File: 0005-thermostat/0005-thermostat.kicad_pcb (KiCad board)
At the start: 2 copper layers, 68.5 x 42 mm, 50 parts, among them J1 EXT_NTC, J2 OUT, J3 PWR, J4 EXT_LED, J5 EXT_P1, J6 EXT_P2, P1 22k, P2 22k, T1 BC847B, T2 BC847B, T3 BC847B

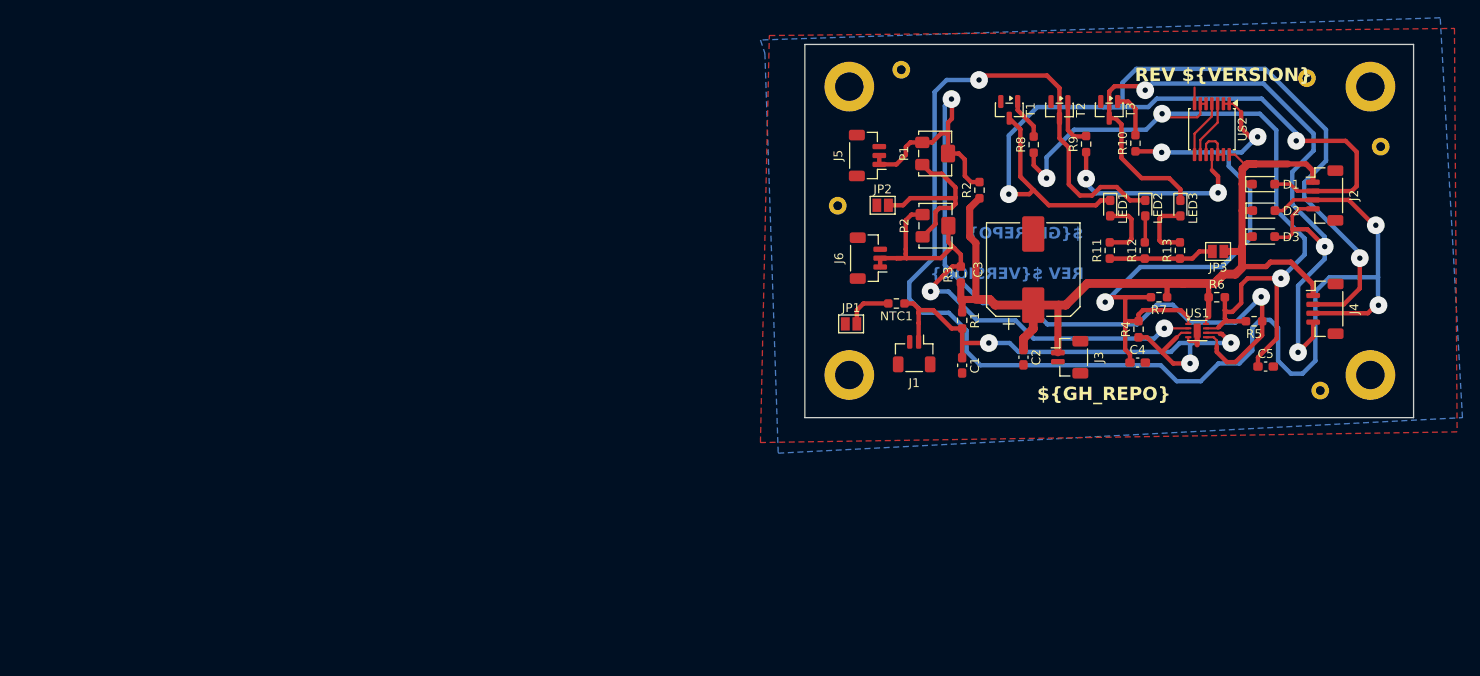
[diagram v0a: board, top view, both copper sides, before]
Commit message: PCB enhancement
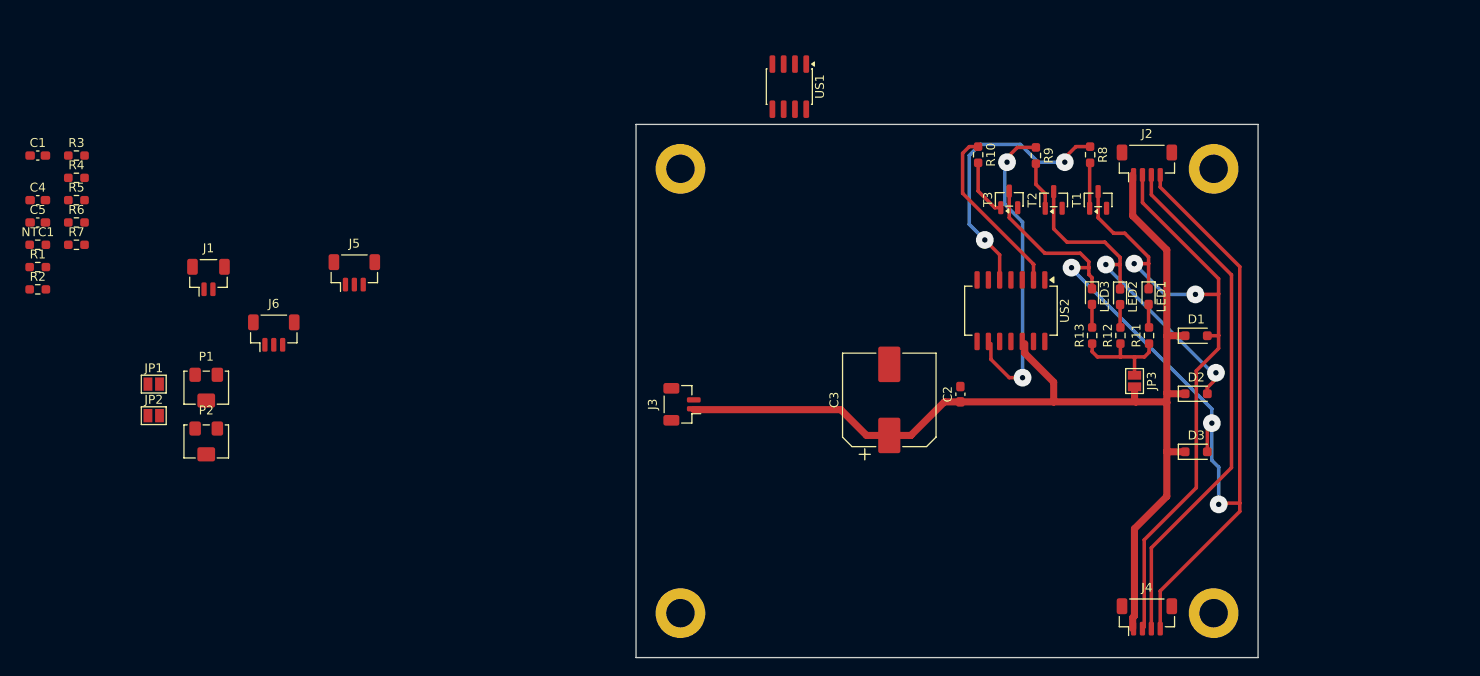
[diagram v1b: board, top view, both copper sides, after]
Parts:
- removed the REF** at (117.7, 89.2)
- removed the REF** at (170.5, 74.8)
- removed the REF** at (172.0, 110.0)
- removed the REF** at (178.8, 82.5)
- removed the REF** at (124.8, 73.8)
- US1: footprint Package_DFN_QFN:DFN-8-1EP_2x2mm_P0.5mm_EP0.8x1.6mm -> Package_SO:SOP-8_3.76x4.96mm_P1.27mm
- US2: footprint Package_SO:TSSOP-14_4.4x5mm_P0.65mm -> Package_SO:SO-14_5.3x10.2mm_P1.27mm
- moved C5 139.1 mm to (27.7, 91.0)
- moved R5 133.2 mm to (32.0, 88.5), turned to 0 degrees
- moved R6 128.6 mm to (32.0, 91.0)
- moved C4 125.1 mm to (27.7, 88.5)
- moved R7 122.0 mm to (32.0, 93.5), turned to 0 degrees
- moved R4 120.7 mm to (32.0, 86.0), turned to 0 degrees
- moved C1 106.7 mm to (27.7, 83.5), turned to 0 degrees
- moved R2 106.6 mm to (27.7, 98.6), turned to 0 degrees
- moved R1 104.2 mm to (27.7, 96.1), turned to 0 degrees
- moved R3 100.4 mm to (32.0, 83.5), turned to 0 degrees
- moved NTC1 96.9 mm to (27.7, 93.5), turned to 0 degrees
- moved P1 86.2 mm to (46.6, 109.6), turned to 0 degrees
- moved P2 85.6 mm to (46.6, 115.7), turned to 0 degrees
- moved JP2 85.4 mm to (40.7, 112.8)
- moved REF** 82.1 mm to (100.0, 135.0)
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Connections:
- J1 pad MP: GNDD -> (no net)
- J3 pad MP: GNDD -> (no net)
- J5 pad MP: GNDD -> (no net)
- J6 pad MP: GNDD -> (no net)
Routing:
- net Net-(J5-Pin_1): track 97.5 -> 0.00 mm, vias 2 -> 0
- net Net-(D2-A): track 166.8 -> 97.4 mm, vias 3 -> 2
- net Net-(J1-Pin_1): track 63.9 -> 0.00 mm, vias 3 -> 0
- net Net-(J6-Pin_1): track 58.4 -> 0.00 mm, vias 2 -> 0
- net Net-(D1-A): track 145.0 -> 87.4 mm, vias 3 -> 2
- net Net-(C5-Pad1): track 88.9 -> 31.5 mm, vias 3 -> 2
- net Net-(C4-Pad1): track 73.1 -> 19.6 mm, vias 3 -> 0
- net Net-(D3-A): track 87.2 -> 117.0 mm
- net Net-(JP2-B): track 20.6 -> 0.00 mm
- net Net-(R9-Pad1): track 23.4 -> 35.6 mm
- net +12V: track 114.6 -> 126.2 mm
- net Net-(JP3-B): track 19.8 -> 12.3 mm
- net Net-(US2-Pad4): track 6.53 -> 0.00 mm
- net Net-(US2-Pad3): track 6.53 -> 0.00 mm
- net GNDD: track 5.98 -> 0.00 mm
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- removed copper zone on B.Cu, net GNDD
- removed copper zone on F.Cu, net GNDD
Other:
- board size 68.5 x 42 mm -> 70 x 60 mm
- board text removed: "${GH_REPO}"
- board text removed: "REV ${VERSION}"
